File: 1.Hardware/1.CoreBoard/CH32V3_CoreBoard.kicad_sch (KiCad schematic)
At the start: 54 parts, among them J2 SH1.0_4P, J3 USB-Type-C, J4 BTB_02X18, J5 BTB_02X18, SW1 3x4, SW2 3x4, SW3 3x4, SW4 3x4, U2 RT9013-33GB, U3 BMI270, U5 IPS096, Y1 32.768KHz, Y2 8MHz

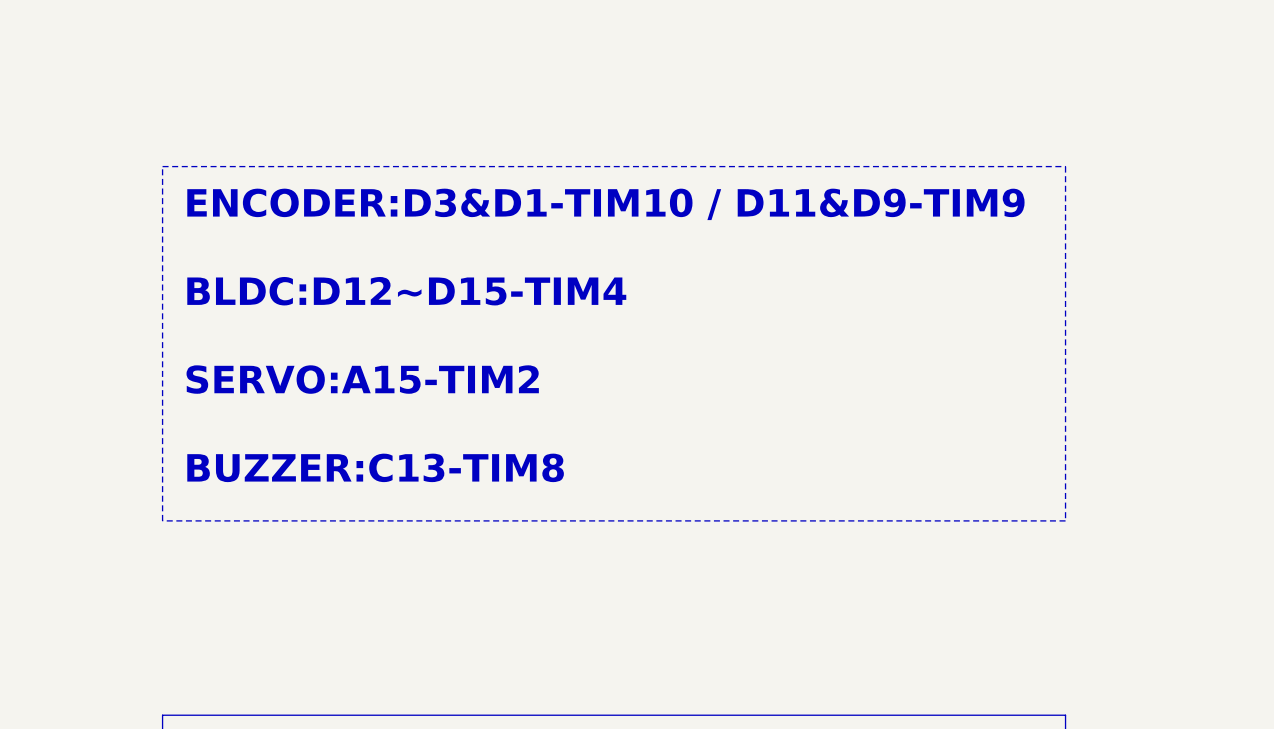
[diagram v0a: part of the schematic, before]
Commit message: MotherBoard finished
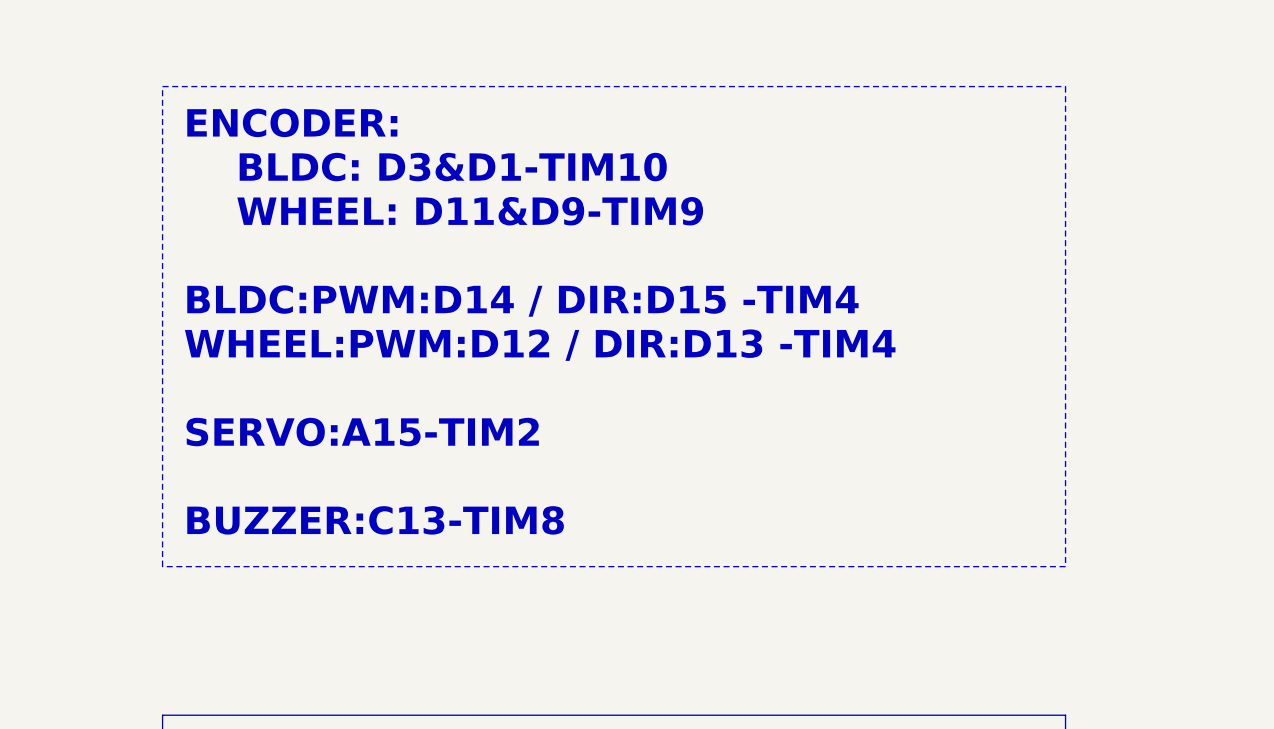
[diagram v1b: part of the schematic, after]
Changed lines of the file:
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@@
     (fill (type none))
   )
-  (text_box "ENCODER:D3&D1-TIM10 / D11&D9-TIM9\n\nBLDC:D12~D15-TIM4\n\nSERVO:A15-TIM2\n\nBUZZER:C13-TIM8"
-    (at 299.72 34.29 0) (size 100.33 39.37)
+  (text_box "ENCODER:\n	BLDC: D3&D1-TIM10\n	WHEEL: D11&D9-TIM9\n\nBLDC:PWM:D14 / DIR:D15 -TIM4\nWHEEL:PWM:D12 / DIR:D13 -TIM4\n\nSERVO:A15-TIM2\n\nBUZZER:C13-TIM8"
+    (at 299.72 25.4 0) (size 100.33 53.34)
     (stroke (width 0.127) (type dash_dot) (color 255 0 0 1))
     (fill (type color) (color 194 194 0 1))
